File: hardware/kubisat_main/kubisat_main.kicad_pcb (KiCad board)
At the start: 2 copper layers, 80 x 80 mm, 37 parts, among them J1 DEBUG_SWD, J2 Micro_SD_Card_Det1, J3 UART0, J4 POWER_IN, J5 IPX, J6 POWER, J7 I2C1, J8 SPI0, Q1 BSS138, Q2 BSS138, SW2 RESET, U1 DS3231M, U3 NEO-6M-GPS, U4 XL1278-SMT, U6 Pico

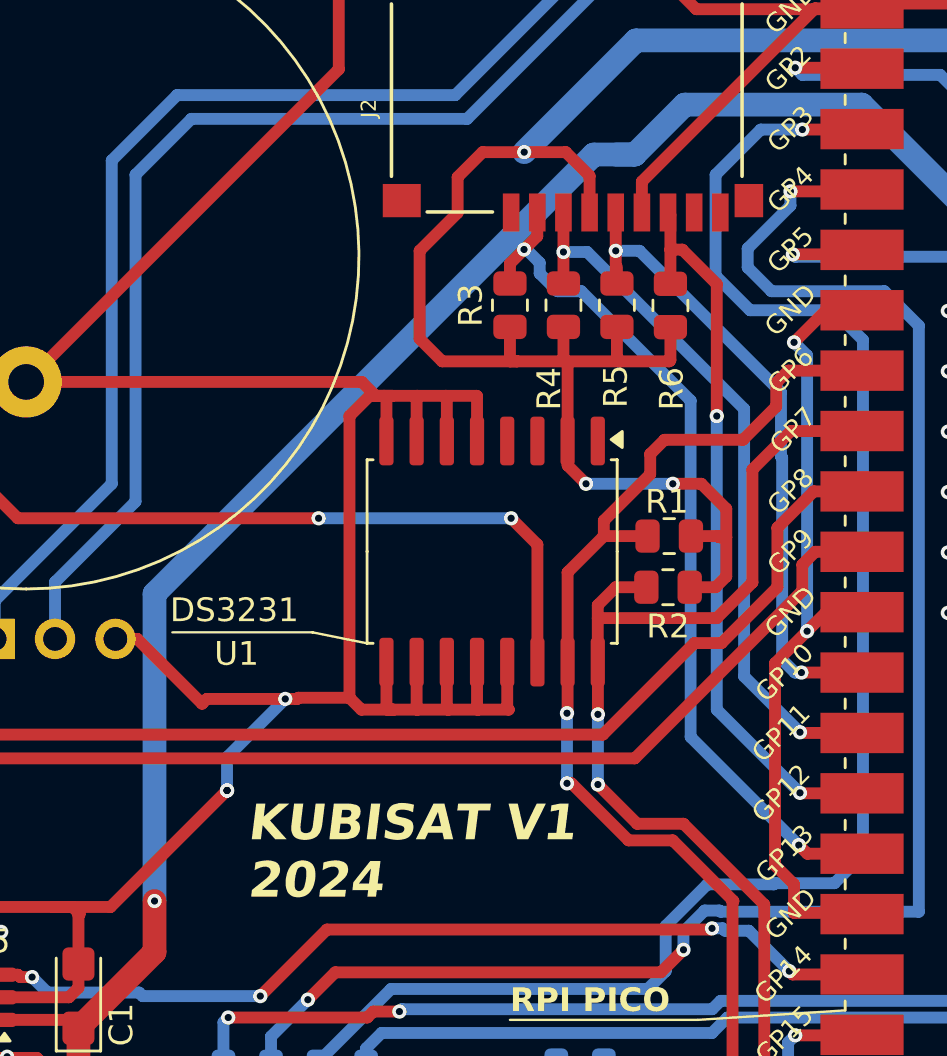
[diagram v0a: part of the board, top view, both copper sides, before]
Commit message: changed folder structure
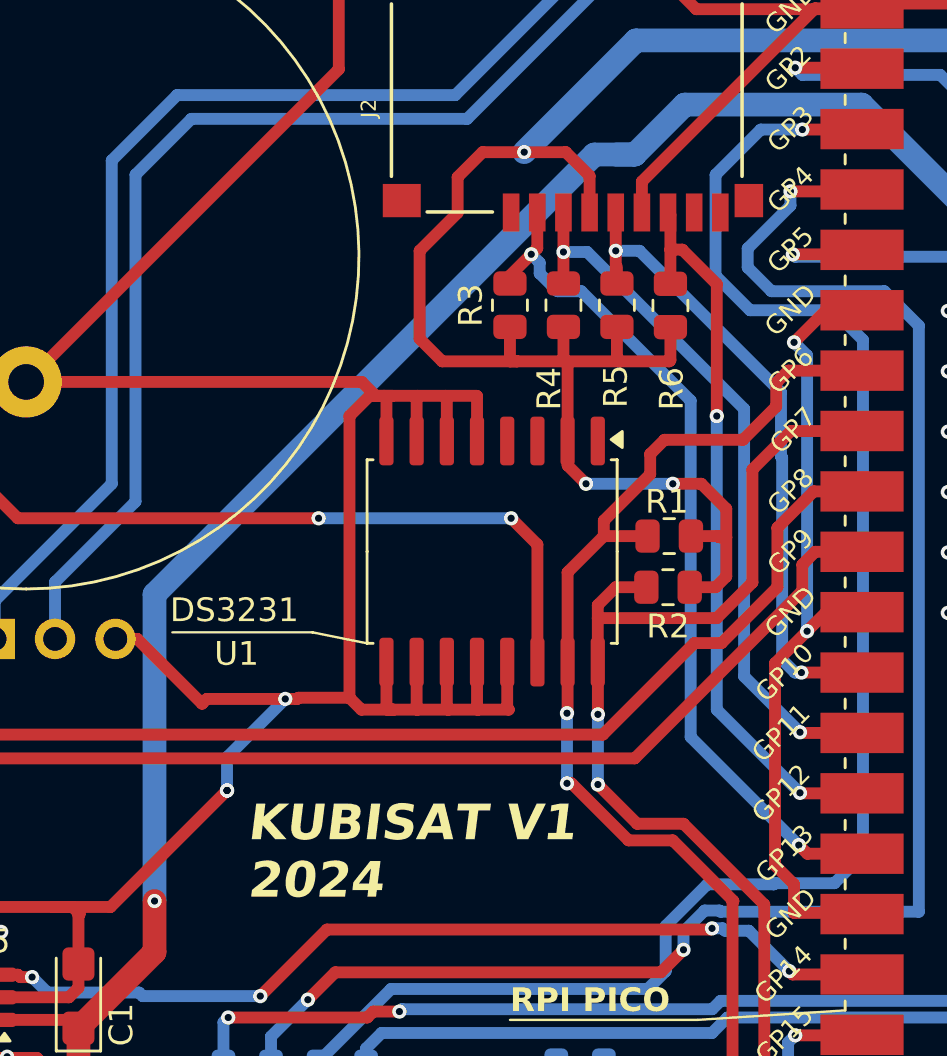
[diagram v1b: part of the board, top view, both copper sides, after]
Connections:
- J2 pad 2: +5V -> SD.CS
- R3 pad 2: +5V -> SD.CS
- U6 pad 17: +5V -> SD.CS
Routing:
- net +5V: track 223.6 -> 185.9 mm, vias 10 -> 8
- net SD.CS: track 0.00 -> 37.3 mm, vias 0 -> 2
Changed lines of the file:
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@@
 	(net 66 "unconnected-(J2-DET-Pad9)")
 	(net 67 "unconnected-(U5-NC-Pad4)")
+	(net 68 "SD.CS")
 	(footprint "RF:XL1278-SMT"
 		(layer "F.Cu")
@@
 			)
 			(layers "F.Cu" "F.Mask")
-			(net 30 "+5V")
+			(net 68 "SD.CS")
 			(pinfunction "GPIO13")
 			(pintype "bidirectional")
@@
 			(layers "F.Cu" "F.Paste" "F.Mask")
 			(roundrect_rratio 0.243902)
-			(net 30 "+5V")
+			(net 68 "SD.CS")
 			(pintype "passive")
 		)
@@
 			(size 0.7 1.6)
 			(layers "F.Cu" "F.Paste" "F.Mask")
-			(net 30 "+5V")
+			(net 68 "SD.CS")
 			(pinfunction "DAT3/CD")
 			(pintype "bidirectional")
@@
 	)
 	(segment
-		(start 77.91 78.71)
-		(end 77.55 78.35)
-		(width 0.5)
-		(layer "F.Cu")
-		(net 30)
-	)
-	(segment
 		(start 68.3625 97.425)
 		(end 69.3125 97.425)
@@
 	)
 	(segment
-		(start 66.55 52.7375)
-		(end 65.99375 53.29375)
-		(width 0.5)
-		(layer "F.Cu")
-		(net 30)
-	)
-	(segment
 		(start 98.9 40.6)
 		(end 98.89 40.61)
@@
 	)
 	(segment
-		(start 81.11 78.71)
-		(end 77.91 78.71)
-		(width 0.5)
-		(layer "F.Cu")
-		(net 30)
-	)
-	(segment
 		(start 71.45 110.45)
 		(end 70.65 110.45)
@@
 	)
 	(segment
-		(start 65.4 53.8875)
-		(end 65.4 54.725)
-		(width 0.5)
-		(layer "F.Cu")
-		(net 30)
-	)
-	(segment
 		(start 58 102.1)
 		(end 58 106.6)
@@
 	)
 	(segment
-		(start 66.55 51.7375)
-		(end 66.55 52.7375)
-		(width 0.5)
-		(layer "F.Cu")
-		(net 30)
-	)
-	(segment
 		(start 69.6 97.7125)
 		(end 69.6 98.925)
@@
 	)
 	(segment
-		(start 65.99375 53.29375)
-		(end 65.4 53.8875)
-		(width 0.5)
-		(layer "F.Cu")
-		(net 30)
-	)
-	(segment
 		(start 68.5375 102.2)
 		(end 67.9625 101.625)
@@
 	)
 	(via
-		(at 77.55 78.35)
-		(size 0.6)
-		(drill 0.3)
-		(layers "F.Cu" "B.Cu")
-		(net 30)
-	)
-	(via
 		(at 47.25 87.85)
 		(size 0.6)
@@
 	)
 	(via
-		(at 65.99375 53.29375)
-		(size 0.6)
-		(drill 0.3)
-		(layers "F.Cu" "B.Cu")
-		(net 30)
-	)
-	(via
 		(at 50.45 80.7)
 		(size 0.6)
@@
 	)
 	(segment
-		(start 66.65 53.85)
-		(end 66.09375 53.29375)
-		(width 0.5)
-		(layer "B.Cu")
-		(net 30)
-	)
-	(segment
 		(start 65.525 97.425)
 		(end 66 97.425)
@@
 	)
 	(segment
-		(start 66.09375 53.29375)
-		(end 65.99375 53.29375)
-		(width 0.5)
+		(start 50.45 80.7)
+		(end 50.45 67.8)
+		(width 1)
 		(layer "B.Cu")
 		(net 30)
@@
 	)
 	(segment
-		(start 90.75 51.7)
-		(end 95 47.45)
+		(start 68.95 49.3)
+		(end 70.65 49.3)
 		(width 1)
 		(layer "B.Cu")
@@
 	)
 	(segment
-		(start 73 59.65)
-		(end 68.4 55.05)
-		(width 0.5)
+		(start 90.75 51.7)
+		(end 95 47.45)
+		(width 1)
 		(layer "B.Cu")
 		(net 30)
@@
 	)
 	(segment
-		(start 77.55 78.35)
-		(end 73 73.8)
-		(width 0.5)
+		(start 50.45 67.8)
+		(end 68.95 49.3)
+		(width 1)
 		(layer "B.Cu")
 		(net 30)
@@
 	)
 	(segment
-		(start 66.65 54.3)
-		(end 66.65 53.85)
-		(width 0.5)
-		(layer "B.Cu")
-		(net 30)
-	)
-	(segment
 		(start 84.55 51.55)
 		(end 84.55 51.7)
@@
 	)
 	(segment
-		(start 50.45 67.776839)
-		(end 68.926839 49.3)
-		(width 1)
-		(layer "B.Cu")
-		(net 30)
-	)
-	(segment
 		(start 69.3125 97.425)
 		(end 75.5625 97.425)
@@
 	)
 	(segment
-		(start 73 73.8)
-		(end 73 59.65)
-		(width 0.5)
-		(layer "B.Cu")
-		(net 30)
-	)
-	(segment
 		(start 80.2 47.2)
 		(end 84.55 51.55)
@@
 	)
 	(segment
-		(start 50.45 80.7)
-		(end 50.45 67.776839)
-		(width 1)
-		(layer "B.Cu")
-		(net 30)
-	)
-	(segment
-		(start 68.926839 49.3)
-		(end 70.65 49.3)
-		(width 1)
-		(layer "B.Cu")
-		(net 30)
-	)
-	(segment
-		(start 67.4 55.05)
-		(end 66.65 54.3)
-		(width 0.5)
-		(layer "B.Cu")
-		(net 30)
-	)
-	(segment
 		(start 48.85 90.15)
 		(end 48.85 99.5)
@@
 	)
 	(segment
-		(start 68.4 55.05)
-		(end 67.4 55.05)
-		(width 0.5)
-		(layer "B.Cu")
-		(net 30)
-	)
-	(segment
 		(start 40 91.75)
 		(end 38.4 90.15)
@@
 		(net 62)
 	)
+	(segment
+		(start 77.91 78.71)
+		(end 77.55 78.35)
+		(width 0.5)
+		(layer "F.Cu")
+		(net 68)
+	)
+	(segment
+		(start 81.11 78.71)
+		(end 77.91 78.71)
+		(width 0.5)
+		(layer "F.Cu")
+		(net 68)
+	)
+	(segment
+		(start 66.296875 53.496875)
+		(end 66.55 53.24375)
+		(width 0.5)
+		(layer "F.Cu")
+		(net 68)
+	)
+	(segment
+		(start 66.296875 53.496875)
+		(end 65.4 54.39375)
+		(width 0.5)
+		(layer "F.Cu")
+		(net 68)
+	)
+	(segment
+		(start 66.55 53.24375)
+		(end 66.55 51.7375)
+		(width 0.5)
+		(layer "F.Cu")
+		(net 68)
+	)
+	(segment
+		(start 65.4 54.39375)
+		(end 65.4 54.725)
+		(width 0.5)
+		(layer "F.Cu")
+		(net 68)
+	)
+	(via
+		(at 77.55 78.35)
+		(size 0.6)
+		(drill 0.3)
+		(layers "F.Cu" "B.Cu")
+		(net 68)
+	)
+	(via
+		(at 66.296875 53.496875)
+		(size 0.6)
+		(drill 0.3)
+		(layers "F.Cu" "B.Cu")
+		(net 68)
+	)
+	(segment
+		(start 66.296875 53.496875)
+		(end 66.65 53.85)
+		(width 0.5)
+		(layer "B.Cu")
+		(net 68)
+	)
+	(segment
+		(start 73 73.8)
+		(end 77.55 78.35)
+		(width 0.5)
+		(layer "B.Cu")
+		(net 68)
+	)
+	(segment
+		(start 66.65 54.3)
+		(end 67.4 55.05)
+		(width 0.5)
+		(layer "B.Cu")
+		(net 68)
+	)
+	(segment
+		(start 68.4 55.05)
+		(end 73 59.65)
+		(width 0.5)
+		(layer "B.Cu")
+		(net 68)
+	)
+	(segment
+		(start 66.65 53.85)
+		(end 66.65 54.3)
+		(width 0.5)
+		(layer "B.Cu")
+		(net 68)
+	)
+	(segment
+		(start 67.4 55.05)
+		(end 68.4 55.05)
+		(width 0.5)
+		(layer "B.Cu")
+		(net 68)
+	)
+	(segment
+		(start 73 59.65)
+		(end 73 73.8)
+		(width 0.5)
+		(layer "B.Cu")
+		(net 68)
+	)
 	(zone
